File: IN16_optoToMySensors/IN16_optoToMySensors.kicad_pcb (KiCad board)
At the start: 2 copper layers, 50 x 50 mm, 13 parts, among them IC1 ATMEGA328-A, P0 CONN_10, P1 CONN_10, P2 ICSP, P3 5VIN, P4 ANT, U1 RFM69HW, U2 74LS151, U3 74LS151, U4 AMS1117

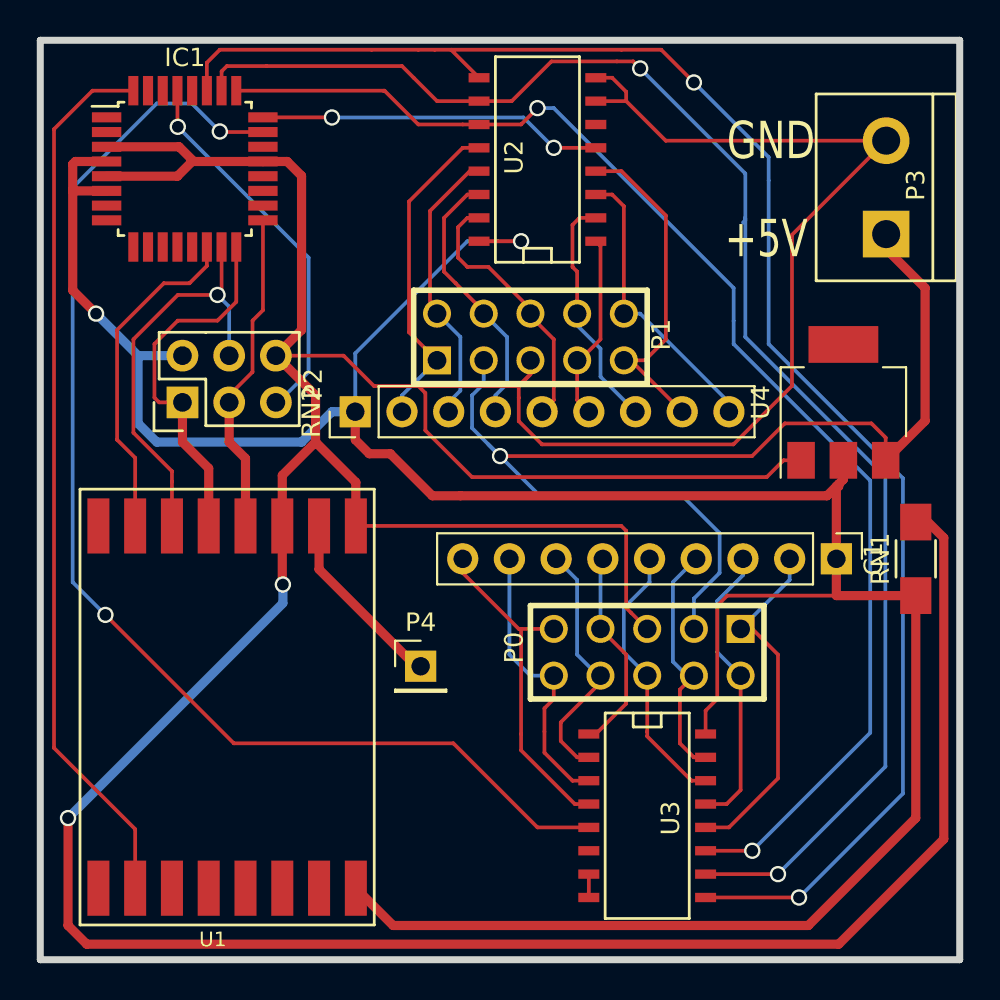
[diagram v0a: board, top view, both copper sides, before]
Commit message: Ajout GERBER
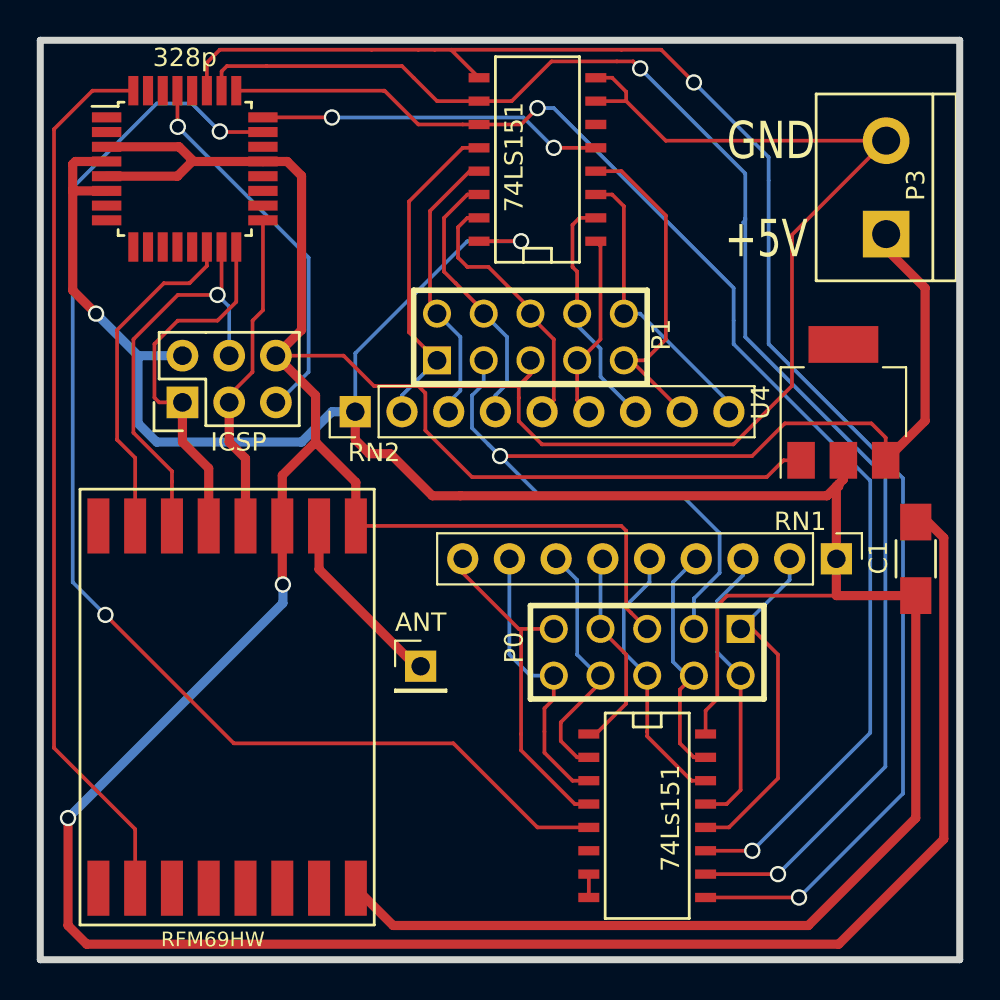
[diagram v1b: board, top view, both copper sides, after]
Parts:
- renumbered IC1 to 328p, U2 to 74LS151, U3 to 74Ls151, P4 to ANT, P2 to ICSP, U1 to RFM69HW
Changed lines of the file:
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@@
   )
   (setup
-    (last_trace_width 0.5)
+    (last_trace_width 0.2032)
     (user_trace_width 0.5)
     (user_trace_width 1.00076)
@@
     (visible_elements FFFFFF7F)
     (pcbplotparams
-      (layerselection 0x00030_80000001)
+      (layerselection 0x010f0_80000001)
       (usegerberextensions true)
       (excludeedgelayer false)
@@
       (psa4output false)
       (plotreference true)
-      (plotvalue false)
+      (plotvalue true)
       (plotinvisibletext false)
       (padsonsilk false)
@@
       (outputformat 1)
       (mirror false)
-      (drillshape 1)
+      (drillshape 0)
       (scaleselection 1)
       (outputdirectory GERBER/))
@@
     (descr "Through hole pin header")
     (tags "pin header")
-    (fp_text reference P2 (at 1.016 7.112 90) (layer F.SilkS)
+    (fp_text reference ICSP (at -2.159 3.048 180) (layer F.SilkS)
       (effects (font (size 1 1) (thickness 0.15)))
     )
@@
     (tags "QFP 0.8")
     (attr smd)
-    (fp_text reference IC1 (at 0 -6.05) (layer F.SilkS)
+    (fp_text reference 328p (at 0 -6.05) (layer F.SilkS)
       (effects (font (size 1 1) (thickness 0.15)))
     )
@@
     (descr RFM69HW)
     (tags "RFM69HW, RF69")
-    (fp_text reference U1 (at -4.191 6.223 180) (layer F.SilkS)
+    (fp_text reference RFM69HW (at -4.191 6.223 180) (layer F.SilkS)
       (effects (font (size 0.8 0.8) (thickness 0.16)))
     )
@@
     (tags "resistor 1206")
     (attr smd)
-    (fp_text reference C1 (at 0 -2.3 90) (layer F.SilkS)
+    (fp_text reference C1 (at 0.0635 -2.032 90) (layer F.SilkS)
       (effects (font (size 1 1) (thickness 0.15)))
     )
@@
     (descr "Through hole straight pin header, 1x01, 2.54mm pitch, single row")
     (tags "Through hole pin header THT 1x01 2.54mm single row")
-    (fp_text reference P4 (at 0 -2.39) (layer F.SilkS)
+    (fp_text reference ANT (at 0 -2.39) (layer F.SilkS)
       (effects (font (size 1 1) (thickness 0.15)))
     )
@@
     (tags "CMS SOJ")
     (attr smd)
-    (fp_text reference U2 (at 0.127 -1.27 90) (layer F.SilkS)
+    (fp_text reference 74LS151 (at 0.127 -1.27 90) (layer F.SilkS)
       (effects (font (size 1 1) (thickness 0.15)))
     )
@@
     (tags "CMS SOJ")
     (attr smd)
-    (fp_text reference U3 (at 0.127 -1.27 270) (layer F.SilkS)
+    (fp_text reference 74Ls151 (at 0.127 -1.27 270) (layer F.SilkS)
       (effects (font (size 1 1) (thickness 0.15)))
     )
@@
     (descr "Through hole straight pin header, 1x09, 2.54mm pitch, single row")
     (tags "Through hole pin header THT 1x09 2.54mm single row")
-    (fp_text reference RN1 (at 0 -2.39 270) (layer F.SilkS)
+    (fp_text reference RN1 (at -2.032 1.9685 360) (layer F.SilkS)
       (effects (font (size 1 1) (thickness 0.15)))
     )
@@
     (descr "Through hole straight pin header, 1x09, 2.54mm pitch, single row")
     (tags "Through hole pin header THT 1x09 2.54mm single row")
-    (fp_text reference RN2 (at 0 -2.39 90) (layer F.SilkS)
+    (fp_text reference RN2 (at -2.2225 1.016 180) (layer F.SilkS)
       (effects (font (size 1 1) (thickness 0.15)))
     )
@@
   (segment (start 134.747 86.487) (end 139.16 90.9) (width 0.2032) (layer Dessus) (net 43))
   (segment (start 134.747 52.832) (end 134.747 86.487) (width 0.2032) (layer Dessus) (net 43))
-  (segment (start 154.686 82.042) (end 154.432 82.042) (width 0.5) (layer Dessus) (net 50) (status C00000))
-  (segment (start 154.432 82.042) (end 149.16 76.77) (width 0.5) (layer Dessus) (net 50) (status 400000))
+  (segment (start 154.686 82.042) (end 154.432 82.042) (width 0.5) (layer Dessus) (net 50))
+  (segment (start 154.432 82.042) (end 149.16 76.77) (width 0.5) (layer Dessus) (net 50))
   (segment (start 149.16 74.41) (end 149.16 76.77) (width 0.5) (layer Dessus) (net 50))
   (segment (start 159.004 70.612) (end 172.708408 70.612) (width 0.2032) (layer Dessus) (net 52))
@@
   (segment (start 182.118 61.468) (end 182.118 68.696) (width 0.5) (layer Dessus) (net 52))
   (segment (start 182.118 68.696) (end 179.973 70.841) (width 0.5) (layer Dessus) (net 52))
-  (segment (start 181.61 78.2) (end 181.61 90.297) (width 0.5) (layer Dessus) (net 53) (status 400000))
+  (segment (start 181.61 78.2) (end 181.61 90.297) (width 0.5) (layer Dessus) (net 53))
   (segment (start 175.768 96.139) (end 153.189 96.139) (width 0.5) (layer Dessus) (net 53))
   (segment (start 181.61 90.297) (end 175.768 96.139) (width 0.5) (layer Dessus) (net 53))
-  (segment (start 177.292 76.2) (end 177.292 72.263) (width 0.5) (layer Dessus) (net 53) (status 400000))
+  (segment (start 177.292 76.2) (end 177.292 72.263) (width 0.5) (layer Dessus) (net 53))
   (segment (start 177.292 72.263) (end 177.419 72.263) (width 0.5) (layer Dessus) (net 53))
   (segment (start 177.419 72.263) (end 177.419 72.136) (width 0.5) (layer Dessus) (net 53))
-  (segment (start 177.292 76.2) (end 177.292 78.2) (width 0.5) (layer Dessus) (net 53) (status 400000))
+  (segment (start 177.292 76.2) (end 177.292 78.2) (width 0.5) (layer Dessus) (net 53))
   (segment (start 177.292 78.2) (end 177.292 78.105) (width 0.2032) (layer Dessus) (net 53))
   (segment (start 177.292 78.105) (end 177.292 78.2) (width 0.2032) (layer Dessus) (net 53))
-  (segment (start 181.61 78.2) (end 177.292 78.2) (width 0.5) (layer Dessus) (net 53) (status 400000))
+  (segment (start 181.61 78.2) (end 177.292 78.2) (width 0.5) (layer Dessus) (net 53))
   (segment (start 177.292 78.2) (end 171.355 78.2) (width 0.2032) (layer Dessus) (net 53))
   (segment (start 170.815 83.82) (end 170.815 78.74) (width 0.2032) (layer Dessus) (net 53))
@@
   (segment (start 170.18 85.725) (end 170.18 84.455) (width 0.2032) (layer Dessus) (net 53))
   (segment (start 171.355 78.2) (end 170.815 78.74) (width 0.2032) (layer Dessus) (net 53))
-  (segment (start 141.732 65.151) (end 139.319 65.151) (width 0.5) (layer Dessous) (net 53) (status 400000))
+  (segment (start 141.732 65.151) (end 139.319 65.151) (width 0.5) (layer Dessous) (net 53))
   (segment (start 139.319 65.151) (end 137.033 62.865) (width 0.5) (layer Dessous) (net 53))
   (via (at 137.033 62.865) (size 0.889) (drill 0.635) (layers Dessus Dessous) (net 53))
   (segment (start 137.033 62.865) (end 135.763 61.595) (width 0.5) (layer Dessus) (net 53))
   (segment (start 135.763 61.595) (end 135.763 56.191) (width 0.5) (layer Dessus) (net 53))
-  (segment (start 151.13 68.199) (end 149.86 68.199) (width 0.5) (layer Dessous) (net 53) (status 400000))
+  (segment (start 151.13 68.199) (end 149.86 68.199) (width 0.5) (layer Dessous) (net 53))
   (segment (start 149.86 68.199) (end 148.209 69.85) (width 0.5) (layer Dessous) (net 53))
   (segment (start 148.209 69.85) (end 140.335 69.85) (width 0.5) (layer Dessous) (net 53))
@@
   (segment (start 135.909 54.591) (end 135.763 54.737) (width 0.5) (layer Dessus) (net 53))
   (segment (start 135.763 54.737) (end 135.763 56.134) (width 0.5) (layer Dessus) (net 53))
-  (segment (start 151.16 74.41) (end 151.16 72.039) (width 0.5) (layer Dessus) (net 54) (status 400000))
+  (segment (start 151.16 74.41) (end 151.16 72.039) (width 0.5) (layer Dessus) (net 54))
   (segment (start 151.16 72.039) (end 148.971 69.85) (width 0.5) (layer Dessus) (net 54))
-  (segment (start 147.16 74.41) (end 147.16 71.661) (width 0.5) (layer Dessus) (net 54) (status 400000))
+  (segment (start 147.16 74.41) (end 147.16 71.661) (width 0.5) (layer Dessus) (net 54))
   (segment (start 147.16 71.661) (end 148.971 69.85) (width 0.5) (layer Dessus) (net 54))
   (segment (start 148.971 69.85) (end 148.971 67.31) (width 0.5) (layer Dessus) (net 54))
-  (segment (start 148.971 67.31) (end 146.812 65.151) (width 0.5) (layer Dessus) (net 54) (status 800000))
+  (segment (start 148.971 67.31) (end 146.812 65.151) (width 0.5) (layer Dessus) (net 54))
   (segment (start 160.655 65.405) (end 160.655 66.167) (width 0.2032) (layer Dessus) (net 54))
   (segment (start 160.655 66.167) (end 160.02 66.802) (width 0.2032) (layer Dessus) (net 54))
